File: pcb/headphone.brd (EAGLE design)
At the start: 94 x 35.6 mm, 30 parts, among them IC101 LF353D, IC201 LF353N, IC301 LF353N, J101 MONOJACKSWITCHCRAFT3, J102 MONOJACKSWITCHCRAFT3, J201 MONOJACKNEUTRIK, J202 MONOJACKNEUTRIK, J301 STEREOJACK, J401 POWER_SIMPLE16, P101 DUALPOT 50K

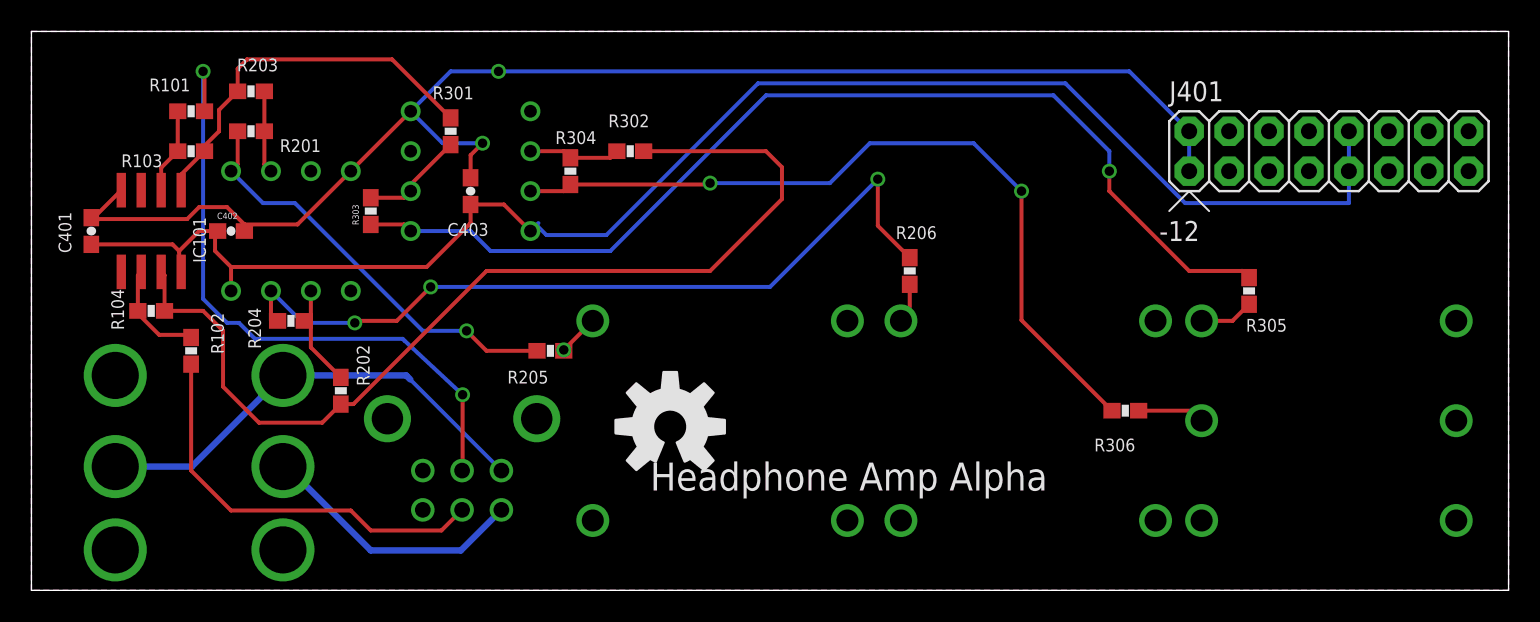
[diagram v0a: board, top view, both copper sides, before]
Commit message: Panel!
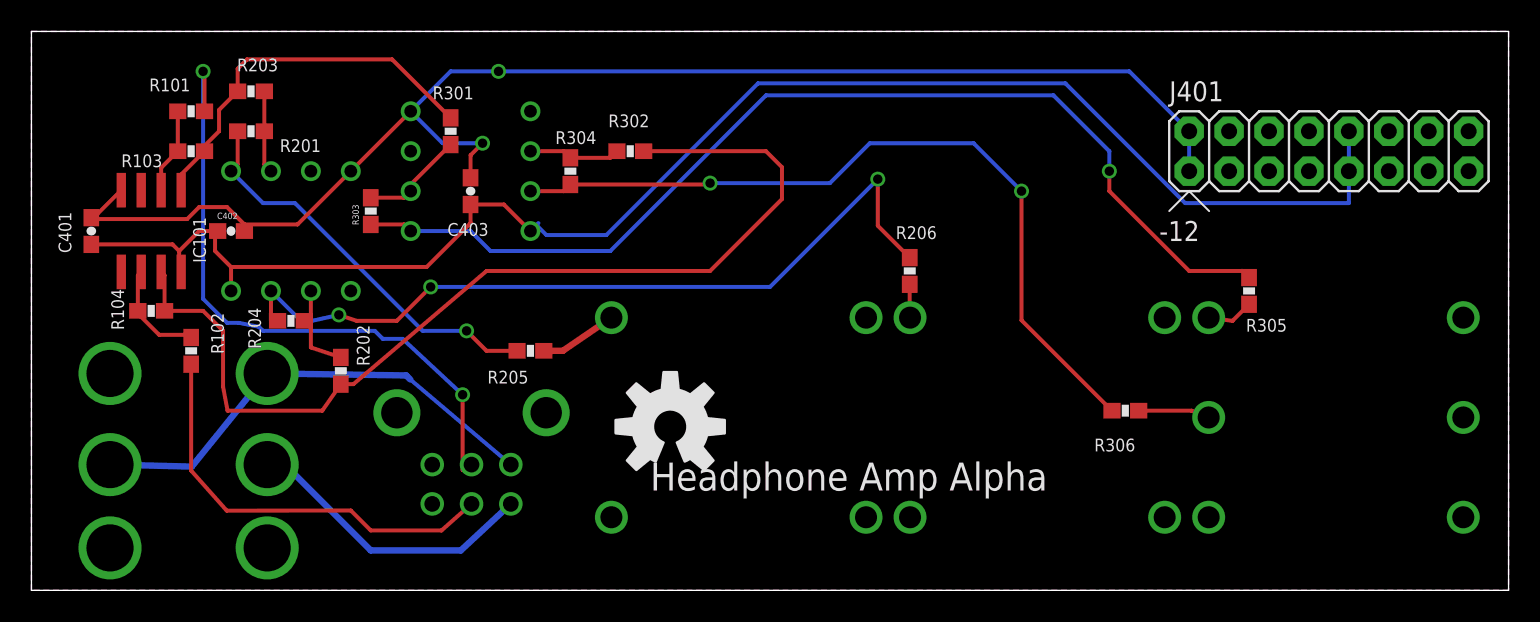
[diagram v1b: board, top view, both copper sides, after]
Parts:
- moved R205 1.27 mm to (31.8, 15.2)
- moved R202 1.27 mm to (19.7, 14.0)
- moved J201 1.20 mm to (45.0, 11.0)
- moved J102 1.01 mm to (15.0, 8.00)
- moved P101 0.71 mm to (28.0, 8.00)
- moved J202 0.62 mm to (64.0, 11.0)
- moved J301 0.49 mm to (83.0, 11.0)
- moved J101 0.36 mm to (5.00, 8.00)
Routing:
- net N$12: track 2.67 -> 4.95 mm, vias 1 -> 0
- net N$3: track 17.2 -> 18.9 mm
- net N$10: track 26.9 -> 25.6 mm
- net J102: track 29.5 -> 30.4 mm
- net N$6: track 26.1 -> 26.9 mm
- net N$8: track 6.71 -> 6.02 mm
- net N$5: track 40.9 -> 41.4 mm
